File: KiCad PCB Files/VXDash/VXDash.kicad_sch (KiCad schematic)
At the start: 82 parts, among them IC1 CD74HC4050M96, J1 Header_VX220_RightAngle, J10 CANbus, J11 LD connector, J12 RD connector, J2 FASCIA PASSTHRU, J5 CAN debug, SW1 RESET, SW2 BOOT, U1 TCA9555PWR, U2 ESP32-S3-WROOM-1

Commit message: Corrected OpAmp routing + more sims
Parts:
- H1: footprint MountingHole:MountingHole_3.7mm_Pad_Via -> MountingHole:MountingHole_3.5mm_Pad_TopOnly
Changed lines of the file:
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@@
 			)
 		)
-		(property "Footprint" "MountingHole:MountingHole_3.7mm_Pad_Via"
+		(property "Footprint" "MountingHole:MountingHole_3.5mm_Pad_TopOnly"
 			(at 27.94 396.24 0)
 			(effects

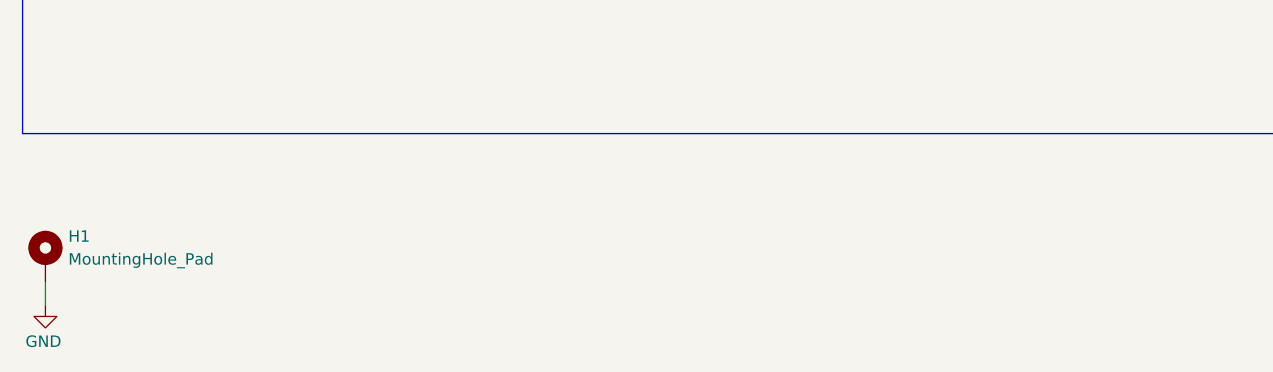
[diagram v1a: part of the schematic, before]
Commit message: New PCB outline
- Corrected small issues with solder expansion mask
- Ground pour in place but no ground stitching
- No Silkscreen texts
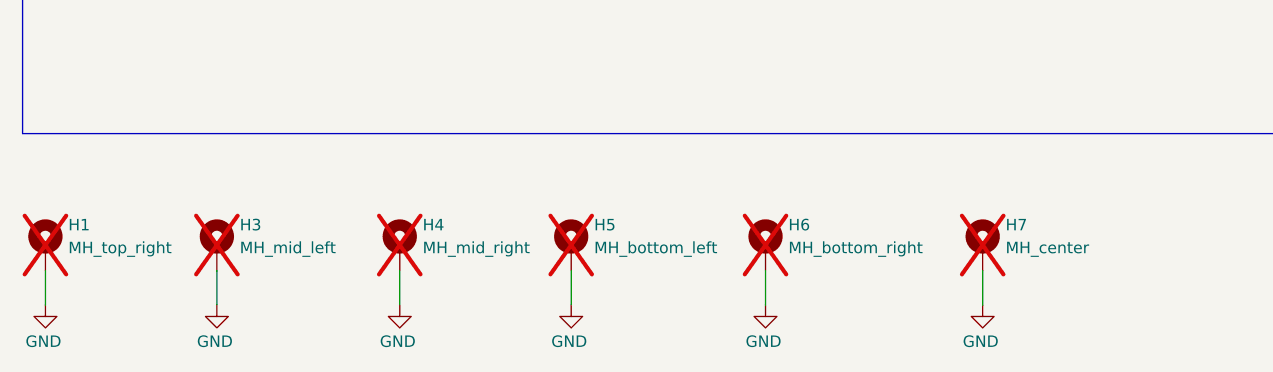
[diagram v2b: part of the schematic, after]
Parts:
- added H3: MH_mid_left, MountingHole:MountingHole_3.5mm_Pad_Via, symbol Mechanical:MountingHole_Pad
- added H4: MH_mid_right, MountingHole:MountingHole_3.5mm_Pad_Via, symbol Mechanical:MountingHole_Pad
- added H5: MH_bottom_left, MountingHole:MountingHole_3.5mm_Pad_Via, symbol Mechanical:MountingHole_Pad
- added H6: MH_bottom_right, MountingHole:MountingHole_3.5mm_Pad_Via, symbol Mechanical:MountingHole_Pad
- added H7: MH_center, MountingHole:MountingHole_3.5mm_Pad_Via, symbol Mechanical:MountingHole_Pad
- H1: value MountingHole_Pad -> MH_top_right; footprint MountingHole:MountingHole_3.5mm_Pad_TopOnly -> MountingHole:MountingHole_3.5mm_Pad_Via; now not fitted
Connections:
- net GND: now also H3.1, H4.1, H5.1, H6.1, H7.1
